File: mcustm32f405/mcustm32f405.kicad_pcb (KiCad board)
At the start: 2 copper layers, 76.2 x 50.8 mm, 31 parts, among them J2 STM32WORLD_BASE, U1 AMS1117-3.3, U2 STM32F405RGTx, U3 SRV05-4, Y1 X_16MHZ

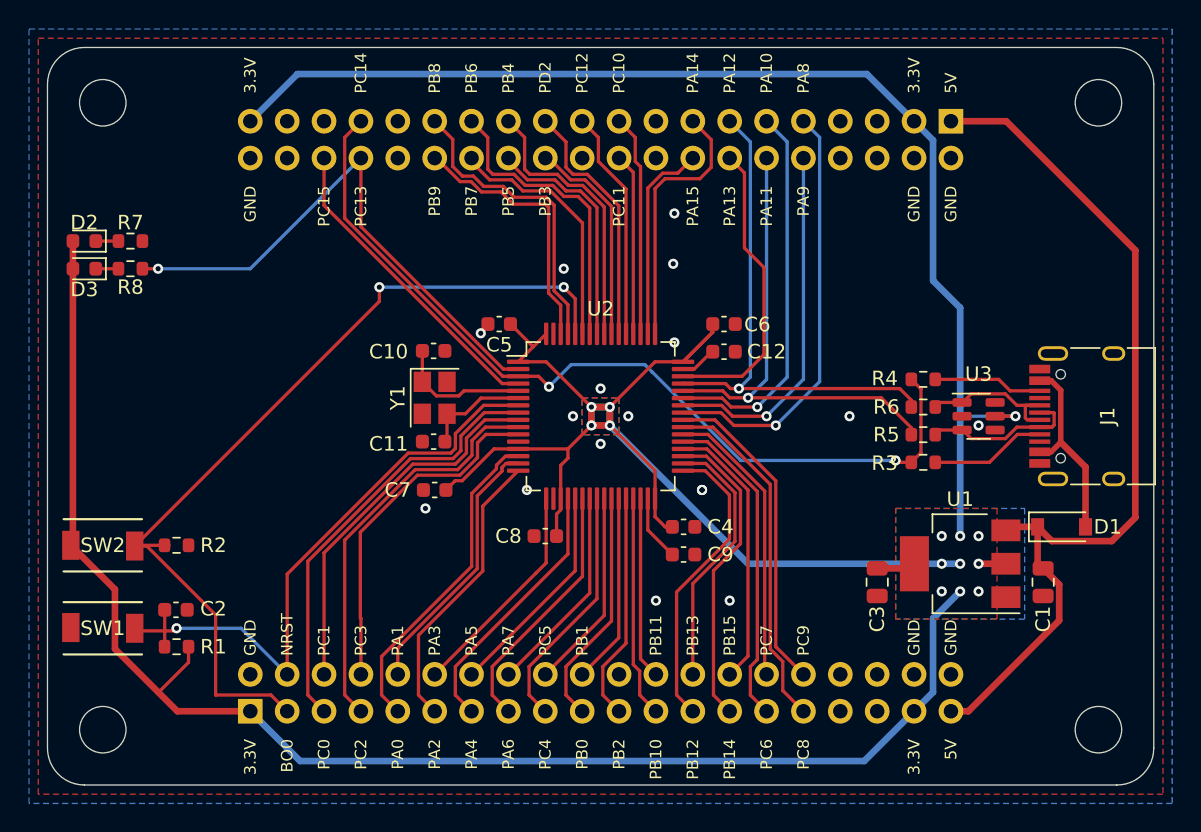
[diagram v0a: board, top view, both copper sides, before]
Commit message: Hmmmm
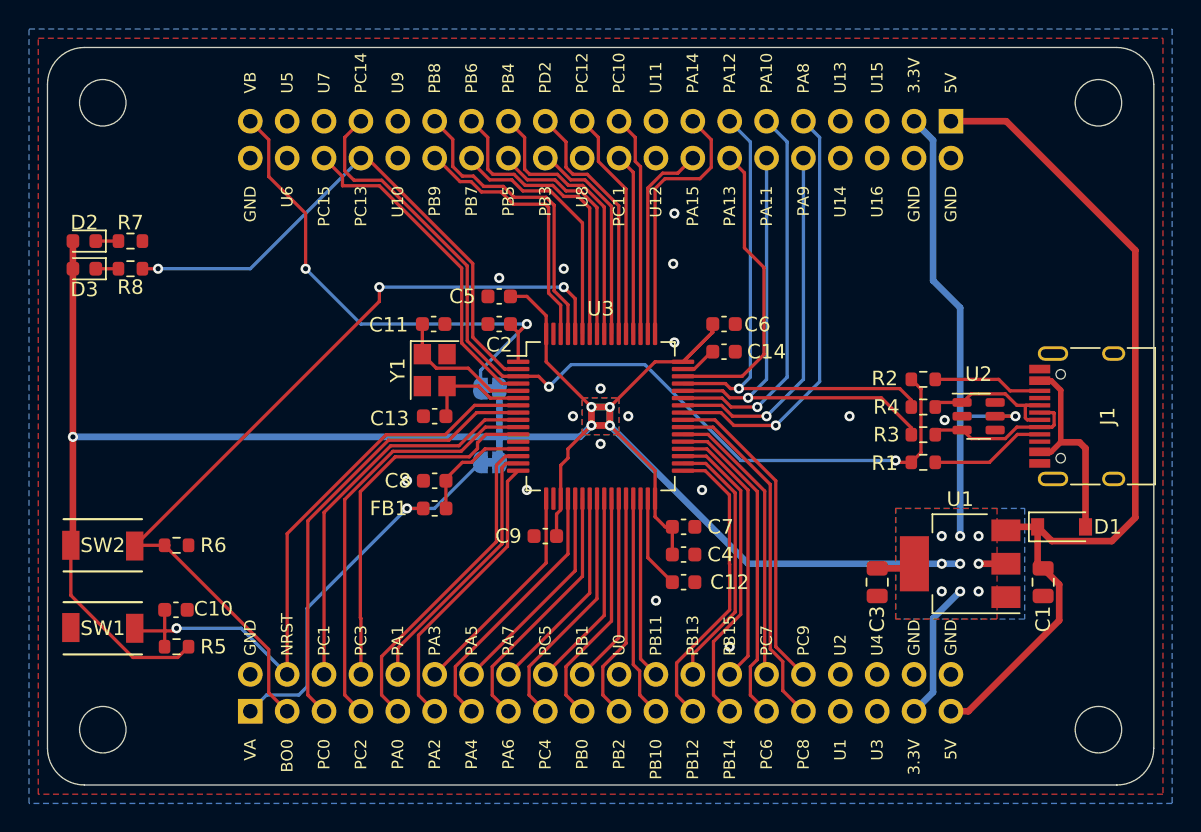
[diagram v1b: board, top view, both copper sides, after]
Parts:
- added C2: C_100NF_0603, Capacitor_SMD:C_0603_1608Metric, F.Cu at (145.4, 95.2)
- added C8: C_100NF_0603, Capacitor_SMD:C_0603_1608Metric, F.Cu at (141.0, 106.0)
- added FB1: FB_0603, Inductor_SMD:L_0603_1608Metric, F.Cu at (141.0, 108.0)
- added JP1: SolderJumper_2_Bridged, Jumper:SolderJumper-2_P1.3mm_Bridged_RoundedPad1.0x1.5mm, B.Cu at (144.8, 99.7)
- added JP2: SolderJumper_2_Bridged, Jumper:SolderJumper-2_P1.3mm_Bridged_RoundedPad1.0x1.5mm, B.Cu at (144.8, 104.8)
- moved C7 17.3 mm to (158.1, 109.2), turned to 0 degrees
- moved C12 1.91 mm to (158.1, 113.0)
- moved C4 1.91 mm to (158.1, 111.1)
- moved C5 1.91 mm to (145.4, 93.3)
- moved Y1 1.91 mm to (141.0, 98.4)
- moved C11 1.85 mm to (140.9, 95.2)
- moved C13 1.75 mm to (141.0, 101.6)
- renumbered C2 to C10, C10 to C11, C9 to C12, C11 to C13, C12 to C14, C8 to C9, R3 to R1, R4 to R2, R5 to R3, R6 to R4, R1 to R5, R2 to R6, U3 to U2, U2 to U3
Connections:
- J2 pad 1: +3V3 -> VDDA
- J2 pad 79: +3V3 -> VBAT
- U3 pad 1: +3V3 -> VBAT
- U3 pad 13: +3V3 -> VA
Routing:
- net +3V3: track 280.8 -> 206.1 mm, vias 14 -> 15
- net VBAT: track 0.00 -> 37.9 mm, vias 0 -> 2
- net VDDA: track 0.00 -> 27.2 mm, vias 0 -> 1
- net VA: track 0.00 -> 7.88 mm
- net BO0: track 61.9 -> 58.3 mm
- net Net-(C12-Pad1): track 4.55 -> 6.46 mm
- net PC15: track 21.7 -> 23.2 mm
- net PC3: track 24.1 -> 25.3 mm
- net PC14: track 60.7 -> 61.8 mm
- net PC2: track 28.0 -> 29.1 mm
- net PC1: track 26.1 -> 27.2 mm
- net PC0: track 30.1 -> 31.2 mm
- net NRST: track 42.7 -> 43.5 mm
- net PA1: track 19.2 -> 18.5 mm
- net VBUS: track 13.6 -> 14.3 mm
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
